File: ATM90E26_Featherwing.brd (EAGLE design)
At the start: 50.8 x 39.4 mm, 56 parts, among them J1 ST-PJ-312, J2 4P-SMD-2.0-90D, J3 4P-SMD-2.0-90D, J4 12V AC, Q1 8.192MHz, U1 ATM90E26, U2 CJT1117-5.0-SOT223

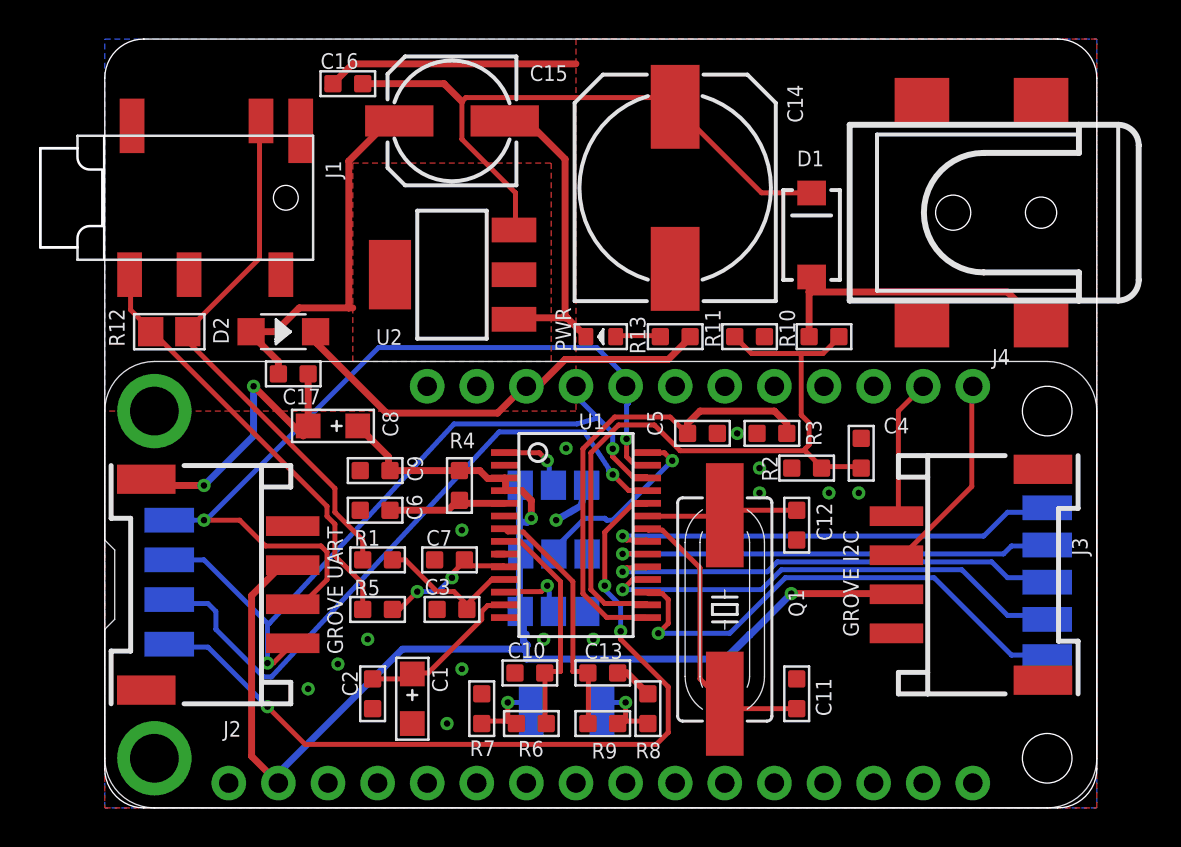
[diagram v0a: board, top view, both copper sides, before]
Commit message: Applied hackvana DRU
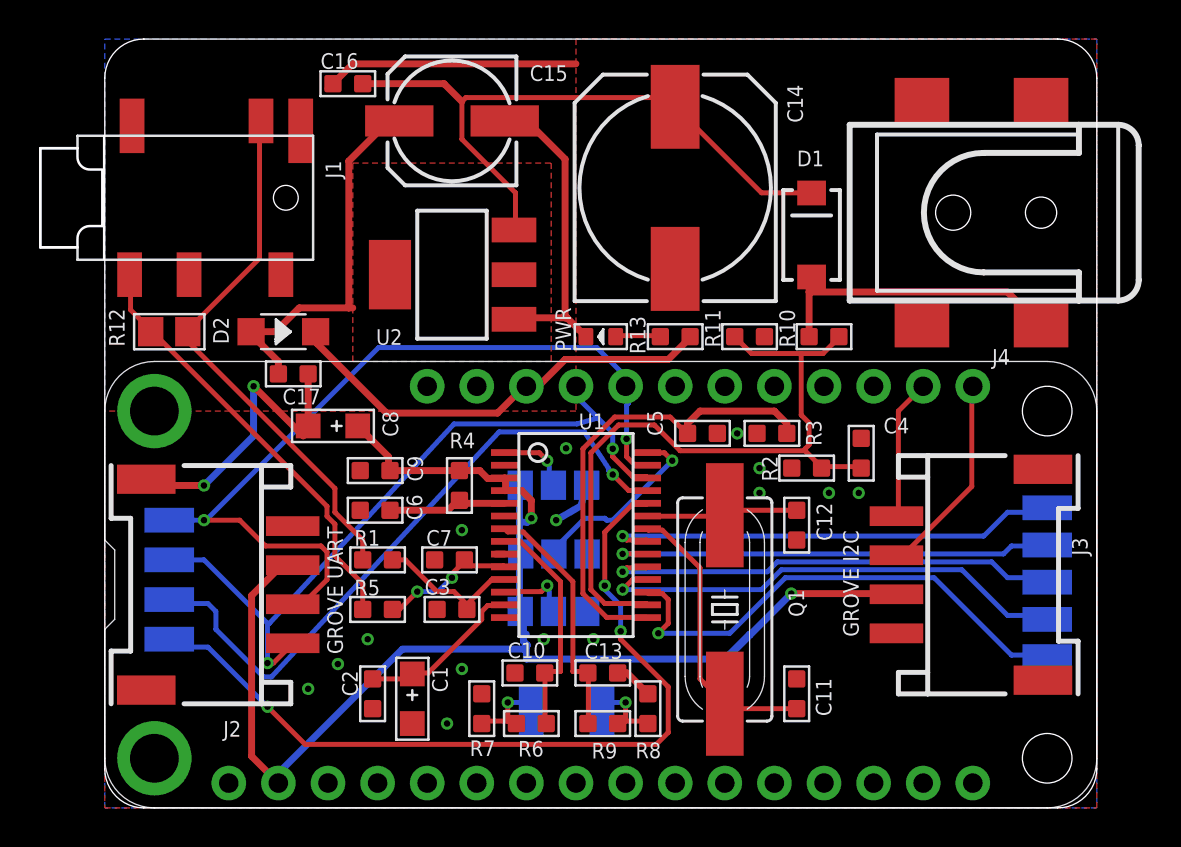
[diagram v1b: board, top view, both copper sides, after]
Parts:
- moved CS 0.25 mm to (3.30, 8.64)
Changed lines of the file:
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@@
 <?xml version="1.0" encoding="utf-8"?>
 <!DOCTYPE eagle SYSTEM "eagle.dtd">
-<eagle version="7.4.0">
+<eagle version="7.6.0">
 <drawing>
 <settings>
@@
 </class>
 </classes>
-<designrules name="OSHPark_2layer">
-<description language="de">&lt;b&gt;EAGLE Design Rules&lt;/b&gt;
+<designrules name="hackvana">
+<description language="de">&lt;b&gt;EAGLE Design Rules für Hackvana&lt;/b&gt;
 &lt;p&gt;
 Die Standard-Design-Rules sind so gewählt, dass sie für
@@
 Einstellungen hier und speichern die Design Rules unter
 einem neuen Namen ab.</description>
-<description language="en">&lt;b&gt;Laen's PCB Order Design Rules&lt;/b&gt;
+<description language="en">&lt;b&gt;EAGLE Design Rules for Hackvana&lt;/b&gt;
 &lt;p&gt;
-Please make sure your boards conform to these design rules.</description>
+The default Design Rules have been set to cover
+a wide range of applications. Your particular design
+may have different requirements, so please make the
+necessary adjustments and save your customized
+design rules under a new name.</description>
+<description language="zh">&lt;b&gt;EAGLE Design Rules for Hackvana&lt;/b&gt;
+</description>
 <param name="layerSetup" value="(1*16)"/>
-<param name="mtCopper" value="0.0356mm 0.0356mm 0.0356mm 0.0356mm 0.0356mm 0.0356mm 0.0356mm 0.0356mm 0.0356mm 0.0356mm 0.0356mm 0.0356mm 0.0356mm 0.0356mm 0.0356mm 0.0356mm"/>
-<param name="mtIsolate" value="1.5011mm 0.1499mm 0.2007mm 0.1499mm 0.2007mm 0.1499mm 0.2007mm 0.1499mm 0.2007mm 0.1499mm 0.2007mm 0.1499mm 0.2007mm 0.1499mm 0.2007mm"/>
+<param name="mtCopper" value="0.035mm 0.035mm 0.035mm 0.035mm 0.035mm 0.035mm 0.035mm 0.035mm 0.035mm 0.035mm 0.035mm 0.035mm 0.035mm 0.035mm 0.035mm 0.035mm"/>
+<param name="mtIsolate" value="1.5mm 0.15mm 0.2mm 0.15mm 0.2mm 0.15mm 0.2mm 0.15mm 0.2mm 0.15mm 0.2mm 0.15mm 0.2mm 0.15mm 0.2mm"/>
 <param name="mdWireWire" value="6mil"/>
 <param name="mdWirePad" value="6mil"/>
@@
 <param name="mdPadVia" value="6mil"/>
 <param name="mdViaVia" value="6mil"/>
-<param name="mdSmdPad" value="6mil"/>
-<param name="mdSmdVia" value="6mil"/>
-<param name="mdSmdSmd" value="6mil"/>
+<param name="mdSmdPad" value="0mil"/>
+<param name="mdSmdVia" value="0mil"/>
+<param name="mdSmdSmd" value="0mil"/>
 <param name="mdViaViaSameLayer" value="8mil"/>
 <param name="mnLayersViaInSmd" value="2"/>
-<param name="mdCopperDimension" value="15mil"/>
+<param name="mdCopperDimension" value="6mil"/>
 <param name="mdDrill" value="6mil"/>
 <param name="mdSmdStop" value="0mil"/>
 <param name="msWidth" value="6mil"/>
-<param name="msDrill" value="13mil"/>
-<param name="msMicroVia" value="13mil"/>
+<param name="msDrill" value="0.3mm"/>
+<param name="msMicroVia" value="0.25mm"/>
 <param name="msBlindViaRatio" value="0.5"/>
 <param name="rvPadTop" value="0.25"/>
@@
 <param name="rvMicroViaOuter" value="0.25"/>
 <param name="rvMicroViaInner" value="0.25"/>
-<param name="rlMinPadTop" value="7mil"/>
+<param name="rlMinPadTop" value="10mil"/>
 <param name="rlMaxPadTop" value="20mil"/>
-<param name="rlMinPadInner" value="7mil"/>
+<param name="rlMinPadInner" value="10mil"/>
 <param name="rlMaxPadInner" value="20mil"/>
-<param name="rlMinPadBottom" value="7mil"/>
+<param name="rlMinPadBottom" value="10mil"/>
 <param name="rlMaxPadBottom" value="20mil"/>
-<param name="rlMinViaOuter" value="7mil"/>
+<param name="rlMinViaOuter" value="6mil"/>
 <param name="rlMaxViaOuter" value="20mil"/>
-<param name="rlMinViaInner" value="7mil"/>
+<param name="rlMinViaInner" value="6mil"/>
 <param name="rlMaxViaInner" value="20mil"/>
 <param name="rlMinMicroViaOuter" value="4mil"/>
@@
 <param name="psTop" value="-1"/>
 <param name="psBottom" value="-1"/>
-<param name="psFirst" value="-1"/>
+<param name="psFirst" value="0"/>
 <param name="psElongationLong" value="100"/>
 <param name="psElongationOffset" value="100"/>
 <param name="mvStopFrame" value="1"/>
 <param name="mvCreamFrame" value="0"/>
-<param name="mlMinStopFrame" value="3mil"/>
-<param name="mlMaxStopFrame" value="3mil"/>
+<param name="mlMinStopFrame" value="2mil"/>
+<param name="mlMaxStopFrame" value="2mil"/>
 <param name="mlMinCreamFrame" value="0mil"/>
 <param name="mlMaxCreamFrame" value="0mil"/>
-<param name="mlViaStopLimit" value="20mil"/>
+<param name="mlViaStopLimit" value="100mil"/>
 <param name="srRoundness" value="0"/>
 <param name="srMinRoundness" value="0mil"/>
@@
 <param name="checkAngle" value="0"/>
 <param name="checkFont" value="1"/>
-<param name="checkRestrict" value="1"/>
+<param name="checkRestrict" value="0"/>
 <param name="useDiameter" value="13"/>
 <param name="maxErrors" value="50"/>
@@
 <attribute name="NAME" x="5.22" y="11.138" size="0.8" layer="26" font="vector" ratio="20" rot="MR180"/>
 </element>
-<element name="CS" library="wirepad" package="SMD1,27-2,54" value="WIREPADSMD1,27-254" x="3.302" y="8.382" smashed="yes" rot="MR90">
-<attribute name="VALUE" x="3.302" y="8.382" size="0.8" layer="28" rot="MR90"/>
-<attribute name="NAME" x="5.474" y="8.852" size="0.8" layer="26" font="vector" ratio="20" rot="MR180"/>
+<element name="CS" library="wirepad" package="SMD1,27-2,54" value="WIREPADSMD1,27-254" x="3.302" y="8.636" smashed="yes" rot="MR90">
+<attribute name="VALUE" x="3.302" y="8.636" size="0.8" layer="28" rot="MR90"/>
+<attribute name="NAME" x="5.474" y="9.106" size="0.8" layer="26" font="vector" ratio="20" rot="MR180"/>
 </element>
 <element name="C16" library="Discrete" package="C0603" value="100n" x="12.446" y="37.084" smashed="yes">
@@
 <wire x1="5.2832" y1="8.2296" x2="8.3312" y2="5.1816" width="0.254" layer="16"/>
 <wire x1="3.4544" y1="8.2296" x2="5.2832" y2="8.2296" width="0.254" layer="16"/>
-<wire x1="3.302" y1="8.382" x2="3.4544" y2="8.2296" width="0.254" layer="16"/>
+<wire x1="3.302" y1="8.636" x2="3.4544" y2="8.2296" width="0.254" layer="16"/>
 <wire x1="27.7368" y1="15.5448" x2="27.786" y2="15.595" width="0.254" layer="1"/>
 <via x="25.6032" y="11.3792" extent="1-16" drill="0.3302"/>
